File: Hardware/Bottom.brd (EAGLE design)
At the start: 120 x 80 mm, 105 parts, among them IC1 OP491SOIC_N14, IC3 74LVC1G17DCK, IC4 LT6231, IC5 SN74CBT3253SOIC16, Q2 25MHz

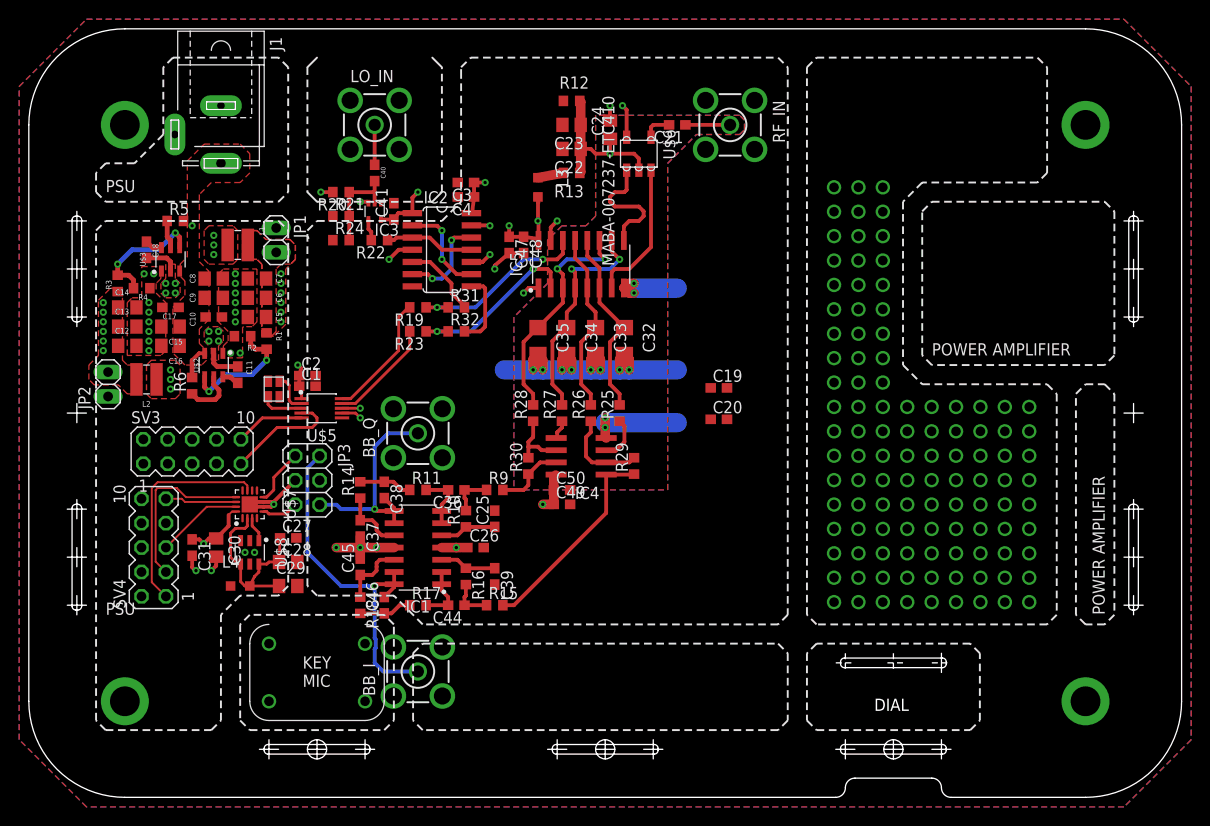
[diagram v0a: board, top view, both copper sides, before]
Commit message: Update board Projektarbeit
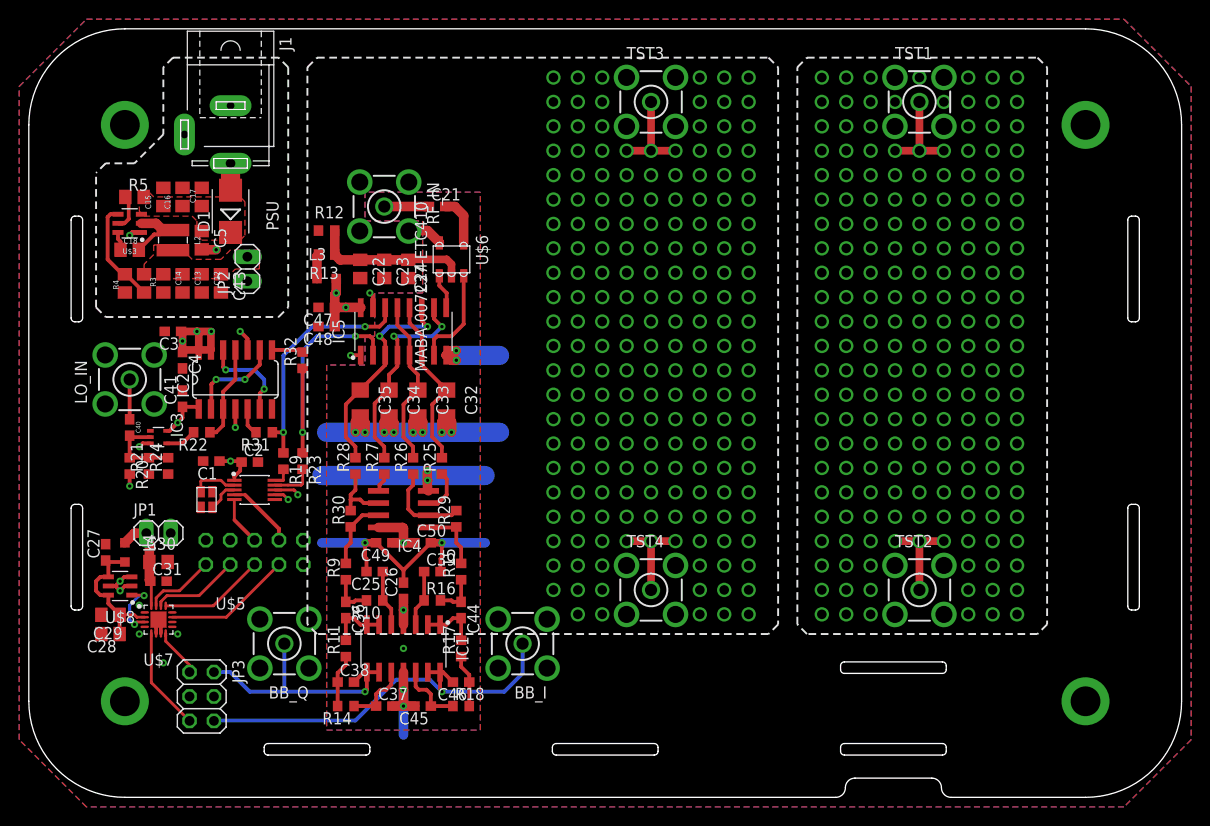
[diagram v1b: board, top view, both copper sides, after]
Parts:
- removed C10, C11, C19, C20: 100n, rcl:C0603
- removed C6, C7: 22µ, rcl:C0805
- removed C8, C9: 4µ7, rcl:C0805
- removed L1: 4.7µH, PowerMagnetics (rev18d):WE-MAPI_3015/3020
- removed R1: 54k9, rcl:R0603
- removed R2, R6: 10k, rcl:R0603
- removed SV3: (no value), con-lstb:MA05-2
- removed U$2: TPS562201, MyLib:SOT95P280X110-6
- added C43: 22µ, rcl:C0805
- added D1: (no value), diode:SMB
- added TST1, TST2, TST3, TST4: BU-SMA-V, con-coax:BU-SMA-V
- C17, C18: device rcl:C0603 -> rcl:C0805
- C5: value 22µ -> 4µ7
- R3, R4, R5: device rcl:R0603 -> rcl:R0805
- moved RF_IN 37.0 mm to (37.0, 61.5)
- moved C40 36.8 mm to (10.5, 38.5)
- moved LO_IN 36.8 mm to (10.5, 43.5), turned to 90 degrees
- moved R20 36.0 mm to (10.5, 34.5), turned to 270 degrees
- moved C3 34.2 mm to (15.0, 48.5)
- moved C4 34.0 mm to (16.0, 45.5), turned to 270 degrees
- moved JP1 32.9 mm to (13.5, 27.5), turned to 0 degrees
- moved R21 32.8 mm to (12.5, 34.5), turned to 90 degrees
- moved IC3 32.5 mm to (13.5, 37.5), turned to 270 degrees
- moved R24 29.6 mm to (14.5, 34.5), turned to 90 degrees
- moved C41 29.4 mm to (16.0, 41.5)
- moved R12 28.9 mm to (31.0, 59.0)
- moved R22 27.2 mm to (18.0, 38.0)
- moved R13 26.9 mm to (31.0, 56.5)
- moved C21 26.4 mm to (42.5, 61.5), turned to 0 degrees
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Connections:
- removed net +5V: JP1.1, SV3.2, SV3.4
- removed net N$11: R1.2, R2.2, U$2.4
- removed net N$30: C5.1, C6.1, C7.1, JP1.2, L1.2, R1.1
- removed net N$35: SV4.10
- removed net N$36: SV4.8
- removed net N$37: SV4.6
- removed net N$38: SV4.4
- removed net N$8: C11.2, L1.1, U$2.2
- removed net RESV_NC: SV4.2
- removed net SPI_MCS_MOSI: SV4.7
- removed net VREG_VDD5_EN: R6.1, U$2.5
- new net FBPEIHRNG: TST3.1
- new net TST1: TST1.1
- new net TST2: TST2.1
- new net TST4: TST4.1
- new net VCCADC: C30.1, C31.1, JP1.1, L4.1, U$7.16
- net +3V3: now also JP1.2, SV4.10, SV4.8; no longer C19.1, C20.1, C30.1, C31.1, SV3.6, SV3.8, U$7.16
- net ADC_CHSEL: now also SV4.3; no longer SV4.1
- net BASEBAND_I: now also JP3.6; no longer JP3.2
- net BASEBAND_Q: now also JP3.2; no longer JP3.6
- net GND: now also C43.2, SV4.1, SV4.2, TST1.2, TST1.3, TST1.4, TST1.5, TST2.2, TST2.3, TST2.4, TST2.5, TST3.2, TST3.3, TST3.4, TST3.5, TST4.2, TST4.3, TST4.4, TST4.5; no longer C10.2, C19.2, C20.2, C6.2, C7.2, C8.2, C9.2, R2.1, SV3.1, SV3.3, SV3.5, SV3.7, U$2.1
- net I2C_MCS_SCL: now also SV4.4; no longer SV3.9
- net I2C_MCS_SDA: now also SV4.6; no longer SV3.10
- net N$31: now also C43.1
- net N$56: now also Q2.3; no longer Q2.4
- net N$7: now also D1.A, J1.3; no longer C11.1, U$2.6
- net SPI_MCS_CLK: now also SV4.7; no longer SV4.9
- net SPI_MCS_CS: now also SV4.5; no longer SV4.3
- net SPI_MCS_MISO: now also SV4.9; no longer SV4.5
- net VDD_DC: now also C5.1, D1.C; no longer C10.1, C8.1, C9.1, J1.3, R6.2, U$2.3
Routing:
- net GND: track 78.3 -> 119.5 mm, vias 43 -> 73
- net +3V3: track 48.2 -> 74.1 mm, vias 13 -> 60
- net N$57: track 21.6 -> 6.93 mm
- net N$11: track 12.9 -> 0.00 mm, vias 2 -> 1
- net N$1: track 13.0 -> 2.05 mm
- net VCCADC: track 0.00 -> 10.4 mm
- net TST4: track 0.00 -> 10.2 mm, vias 0 -> 3
- net TST2: track 0.00 -> 10.2 mm, vias 0 -> 3
- net TST1: track 0.00 -> 10.2 mm, vias 0 -> 3
- net FBPEIHRNG: track 0.00 -> 10.1 mm, vias 0 -> 3
- net ADC_CHSEL: track 22.7 -> 13.4 mm
- net N$51: track 13.0 -> 3.65 mm
- net CLK_Q: track 18.6 -> 27.0 mm
- net N$9: track 7.50 -> 0.00 mm, vias 0 -> 1
- net N$32: track 3.79 -> 10.8 mm
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- added copper zone on layer 1, net NOFILL
- added copper zone on layer 15, net NOFILL
- added copper zone on layer 16, net NOFILL
- added copper zone on layer 2, net NOFILL
- removed copper zone on layer 1, net CUTOUT
- removed copper zone on layer 15, net CUTOUT
- removed copper zone on layer 16, net CUTOUT
- removed copper zone on layer 2, net CUTOUT
- removed copper zone on layer 1, net N$19
- removed copper zone on layer 2, net N$19
- removed copper zone on layer 1, net N$30
- removed copper zone on layer 1, net N$8
- removed copper zone on layer 2, net N$8
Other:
- outline, holes or cut-outs redrawn
- board text added: "+3V3"
- board text added: "GND"
